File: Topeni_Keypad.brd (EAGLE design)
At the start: 31 parts

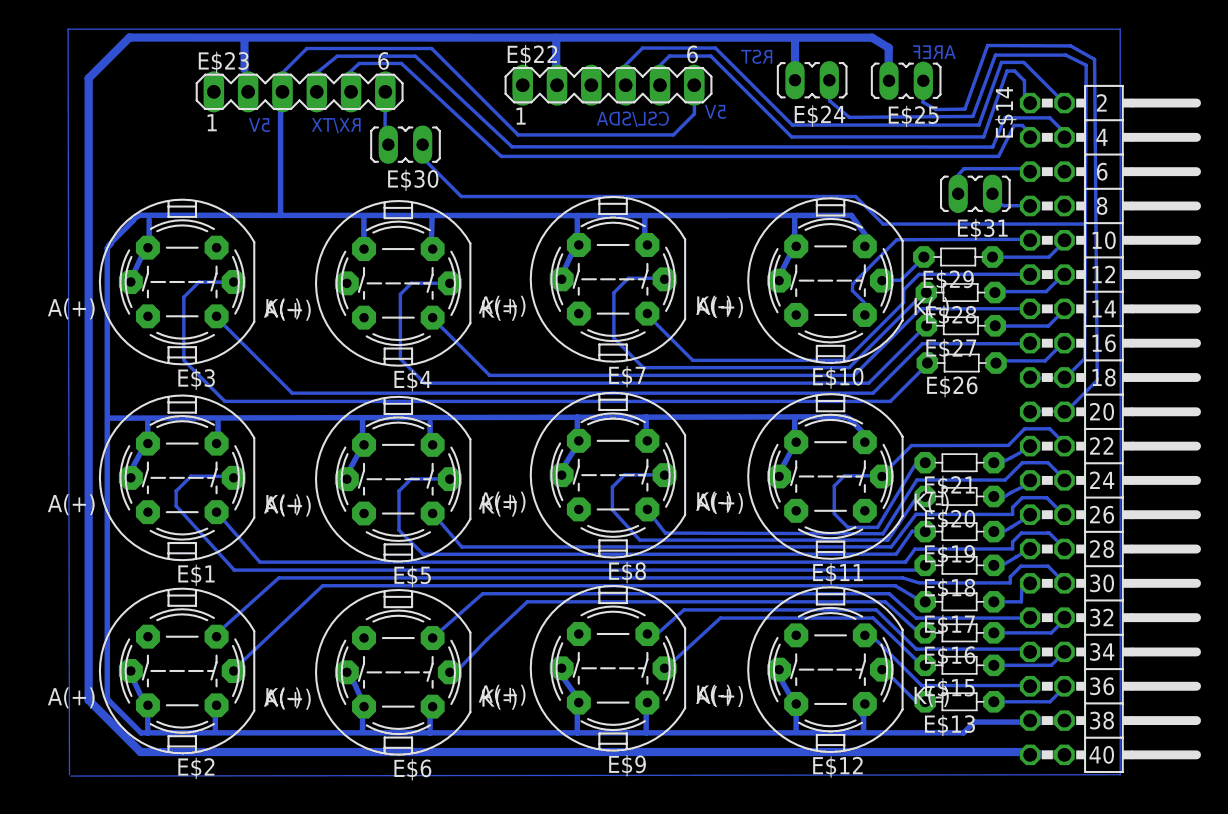
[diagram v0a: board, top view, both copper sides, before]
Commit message: Update + sensors
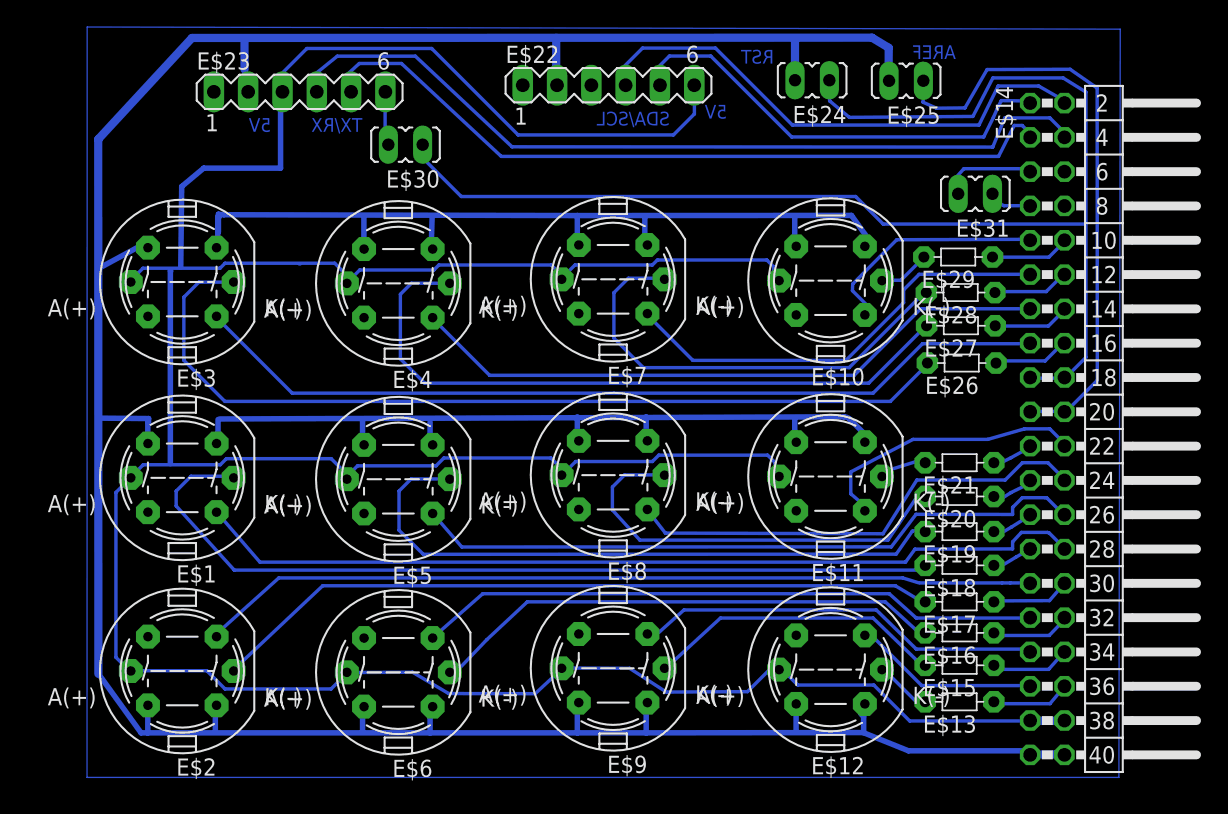
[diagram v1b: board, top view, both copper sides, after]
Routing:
- net S$60: track 179.1 -> 102.9 mm
- net S$23: track 1.70 -> 18.8 mm
- net S$20: track 1.48 -> 16.6 mm
- net S$17: track 1.53 -> 16.4 mm
- net S$25: track 1.66 -> 16.5 mm
- net S$29: track 1.66 -> 16.4 mm
- net S$14: track 1.70 -> 16.3 mm
- net S$27: track 1.57 -> 16.0 mm
- net S$94: track 0.00 -> 14.3 mm
- net S$8: track 1.66 -> 15.8 mm
- net S$9: track 1.97 -> 15.7 mm
- net S$10: track 2.08 -> 15.6 mm
- net S$11: track 1.84 -> 14.1 mm
- net S$56: track 14.4 -> 2.12 mm
- net S$86: track 7.95 -> 18.2 mm
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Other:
- board text added: "SDA/SCL"
- board text added: "TX/RX"
- board text removed: "CSL/SDA"
- board text removed: "RX/TX"
